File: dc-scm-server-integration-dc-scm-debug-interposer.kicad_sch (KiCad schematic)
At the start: 8 parts

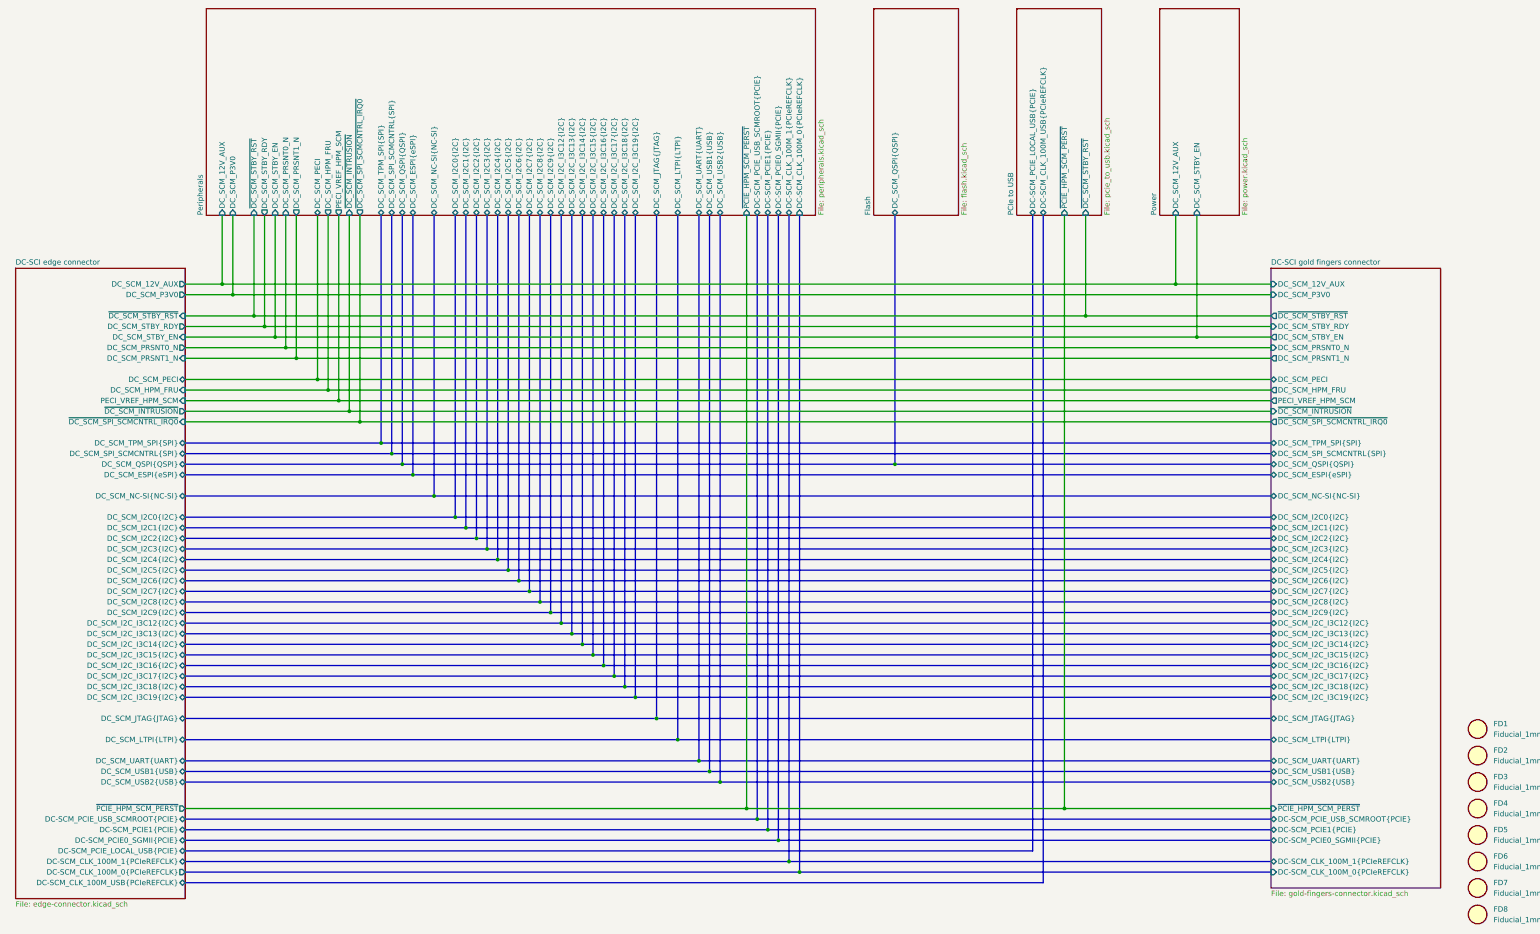
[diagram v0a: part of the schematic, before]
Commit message: [#100720] Clear ERC
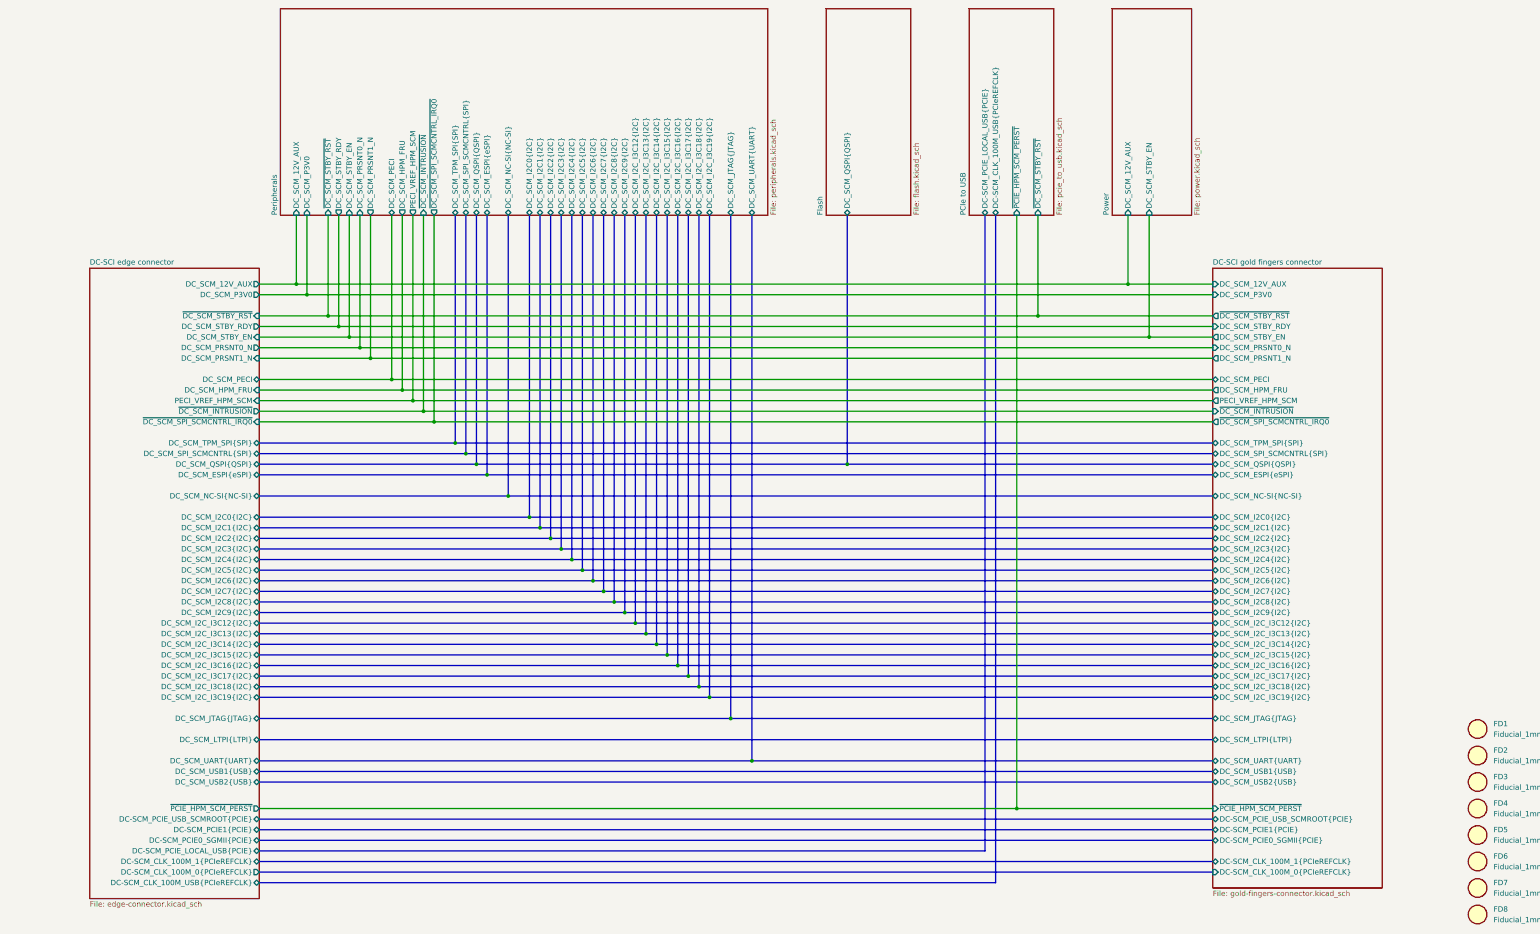
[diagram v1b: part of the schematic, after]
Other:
- sheet Peripherals ports: added none; removed DC-SCM_CLK_100M_0{PCIeREFCLK}, DC-SCM_CLK_100M_1{PCIeREFCLK}, DC-SCM_PCIE0_SGMII{PCIE}, DC-SCM_PCIE1{PCIE}, DC-SCM_PCIE_USB_SCMROOT{PCIE}, DC_SCM_LTPI{LTPI}, DC_SCM_USB1{USB}, DC_SCM_USB2{USB}, ~{PCIE_HPM_SCM_PERST}
